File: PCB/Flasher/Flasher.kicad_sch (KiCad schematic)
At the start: 62 parts, among them J1 Reset, J2 RJ12, J3 USB, J4 USB-C-Socket-V, J5 TF_PUSH, SW1 SW_Push_DPDT, U1 ESP32-S3-MINI-1, U2 TPS562246, U3 FT231XQ, U4 TPS22916CNYFPR, U5 TPS22916CNYFPR

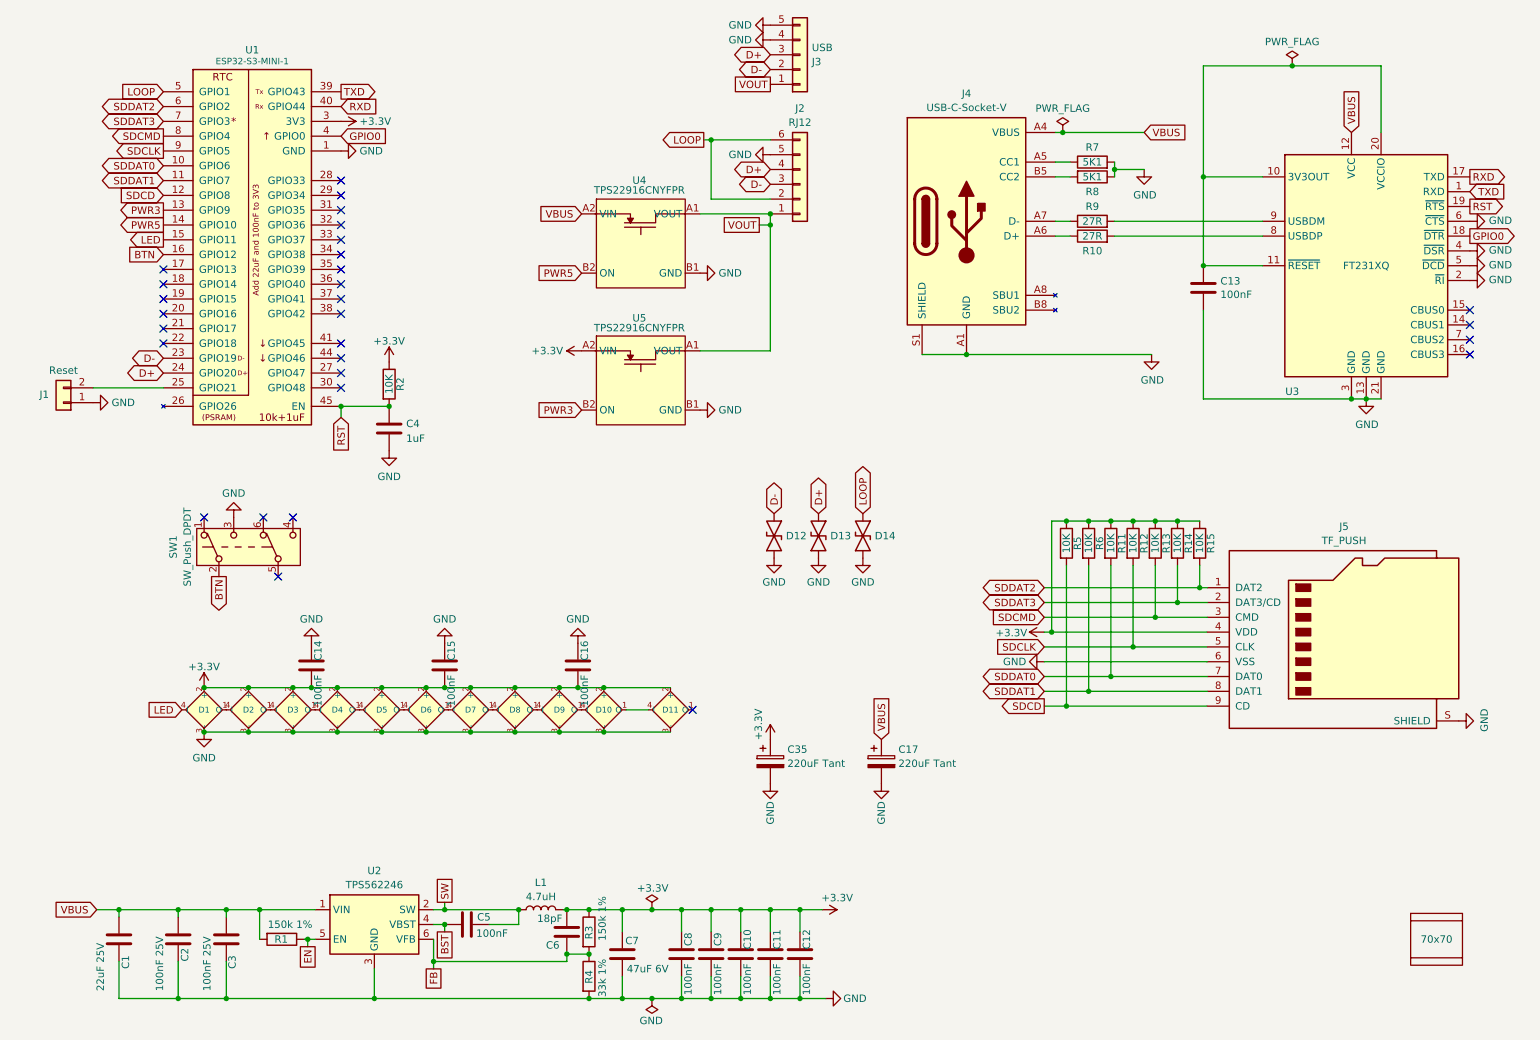
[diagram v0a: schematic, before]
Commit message: LED update
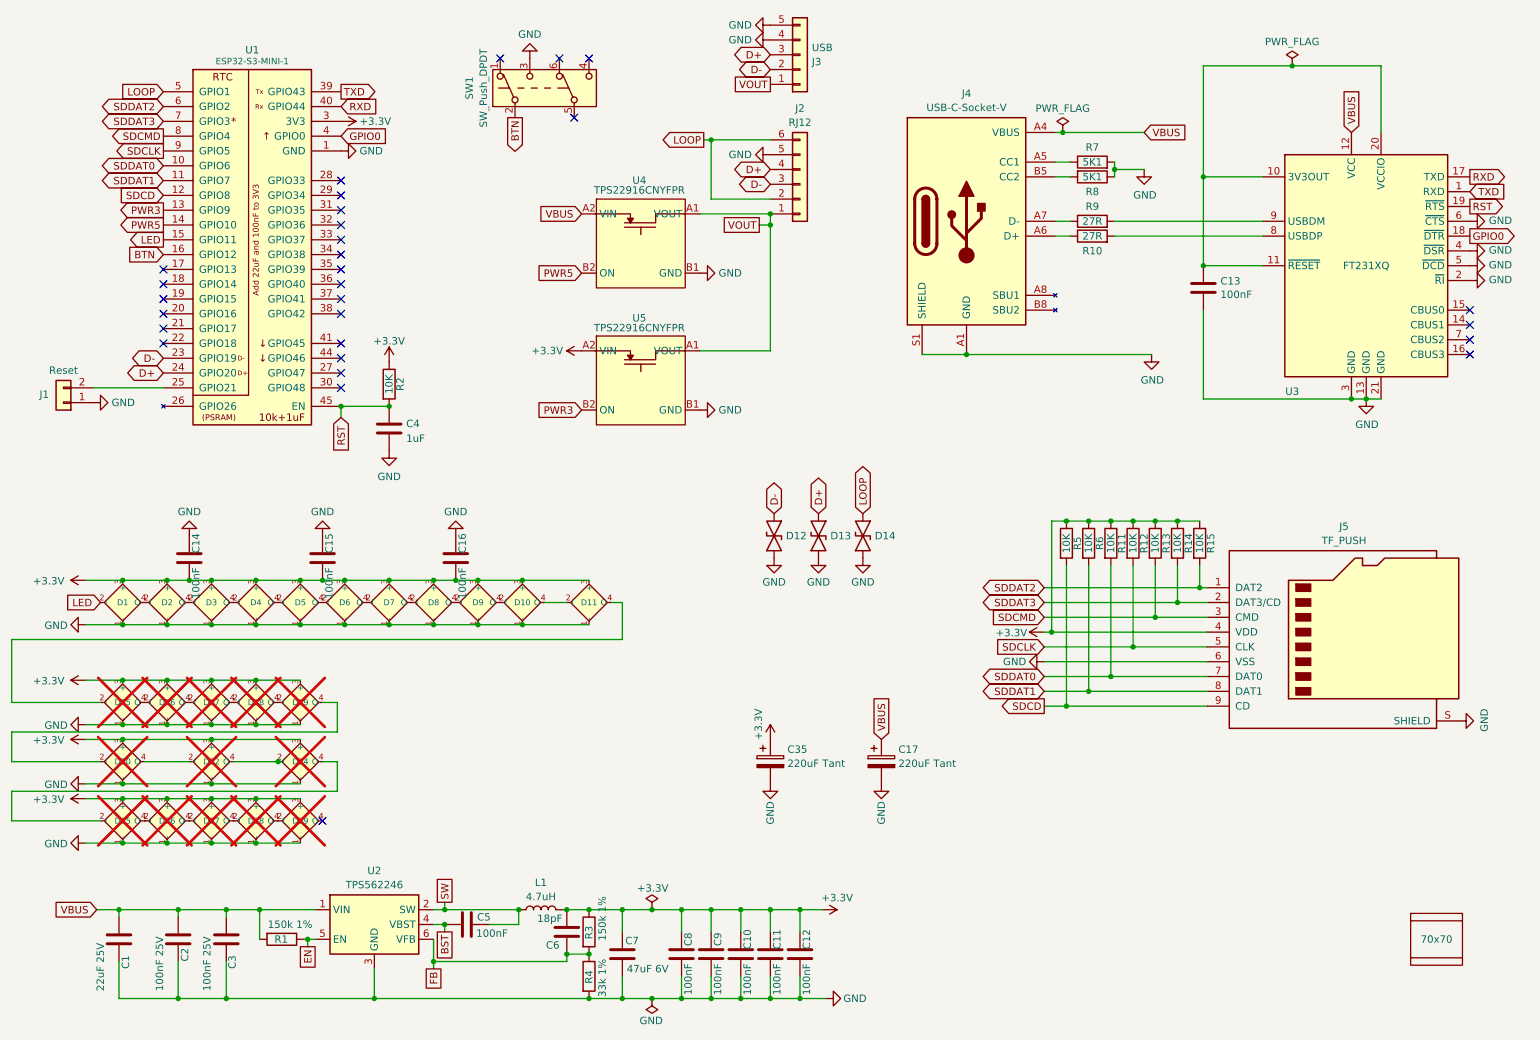
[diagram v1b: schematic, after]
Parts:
- added D15, D16, D17, D18, D19, D20, D22, D24, D25, D26, D27, D28, D29: XL-1010RGBC-WS2812B, RevK:SMD1615, symbol RevK:WS2812B-1.5mm
- D1, D10, D11, D2, D3, D4, D5, D6, D7, D8, D9: footprint RevK:SMD1010 -> RevK:SMD1615; symbol RevK:WS2812B-1mm -> RevK:WS2812B-1.5mm; MPN C5349953 -> C5349954
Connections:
- net +3.3V: now also D1.3 (+), D10.3 (+), D11.3 (+), D2.3 (+), D3.3 (+), D4.3 (+), D5.3 (+), D6.3 (+), D7.3 (+), D8.3 (+), D9.3 (+), D15.3 (+), D16.3 (+), D17.3 (+), D18.3 (+), D19.3 (+), D20.3 (+), D22.3 (+), D24.3 (+), D25.3 (+), D26.3 (+), D27.3 (+), D28.3 (+), D29.3 (+); no longer D1.2 (+), D10.2 (+), D11.2 (+), D2.2 (+), D3.2 (+), D4.2 (+), D5.2 (+), D6.2 (+), D7.2 (+), D8.2 (+), D9.2 (+)
- net GND: now also D1.1 (-), D10.1 (-), D11.1 (-), D2.1 (-), D3.1 (-), D4.1 (-), D5.1 (-), D6.1 (-), D7.1 (-), D8.1 (-), D9.1 (-), D15.1 (-), D16.1 (-), D17.1 (-), D18.1 (-), D19.1 (-), D20.1 (-), D22.1 (-), D24.1 (-), D25.1 (-), D26.1 (-), D27.1 (-), D28.1 (-), D29.1 (-); no longer D1.3 (-), D10.3 (-), D11.3 (-), D2.3 (-), D3.3 (-), D4.3 (-), D5.3 (-), D6.3 (-), D7.3 (-), D8.3 (-), D9.3 (-)
- net LED: now also D1.2 (I); no longer D1.4 (I)
- net at D6.4 (O): now also D7.2 (I); no longer D5.1 (O)
- net at D5.4 (O): now also D6.2 (I); no longer D4.1 (O)
- net at D7.4 (O): now also D8.2 (I); no longer D6.1 (O)
- net at D11.4 (O): now also D15.2 (I); no longer D10.1 (O)
- net at D10.4 (O): now also D11.2 (I); no longer D9.1 (O)
- net at D3.4 (O): now also D4.2 (I); no longer D2.1 (O)
- net at D2.4 (O): now also D3.2 (I); no longer D1.1 (O)
- net at D8.4 (O): now also D9.2 (I); no longer D7.1 (O)
- net at D4.4 (O): now also D5.2 (I); no longer D3.1 (O)
- net at D9.4 (O): now also D10.2 (I); no longer D8.1 (O)
- new net: D27.4 (O), D28.2 (I)
- new net: D28.4 (O), D29.2 (I)
- new net: D16.4 (O), D17.2 (I)
- new net: D17.4 (O), D18.2 (I)
- new net: D1.4 (O), D2.2 (I)
- new net: D22.4 (O), D24.2 (I)
- new net: D24.4 (O), D25.2 (I)
- new net: D26.4 (O), D27.2 (I)
- new net: D25.4 (O), D26.2 (I)
- new net: D19.4 (O), D20.2 (I)
- new net: D20.4 (O), D22.2 (I)
- new net: D15.4 (O), D16.2 (I)
- new net: D18.4 (O), D19.2 (I)
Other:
- moved on the sheet: C14, C15, C16, D1, D10, D11, D2, D3, D4, D5, D6, D7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
